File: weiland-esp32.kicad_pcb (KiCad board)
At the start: 2 copper layers, 20.2 x 58 mm, 22 parts, among them J1 S02B-PASK-2, J2 20021221-00006T4LF, J3 S02B-PASK-2, J4 S02B-PASK-2, J6 S02B-PASK-2, J7 S02B-PASK-2, U1 ESP32-WROOM-32E(8MB), U2 AMS1117-3.3_C347222, U3 GR6205-SOP-8, U4 MAX98357AEWL_T

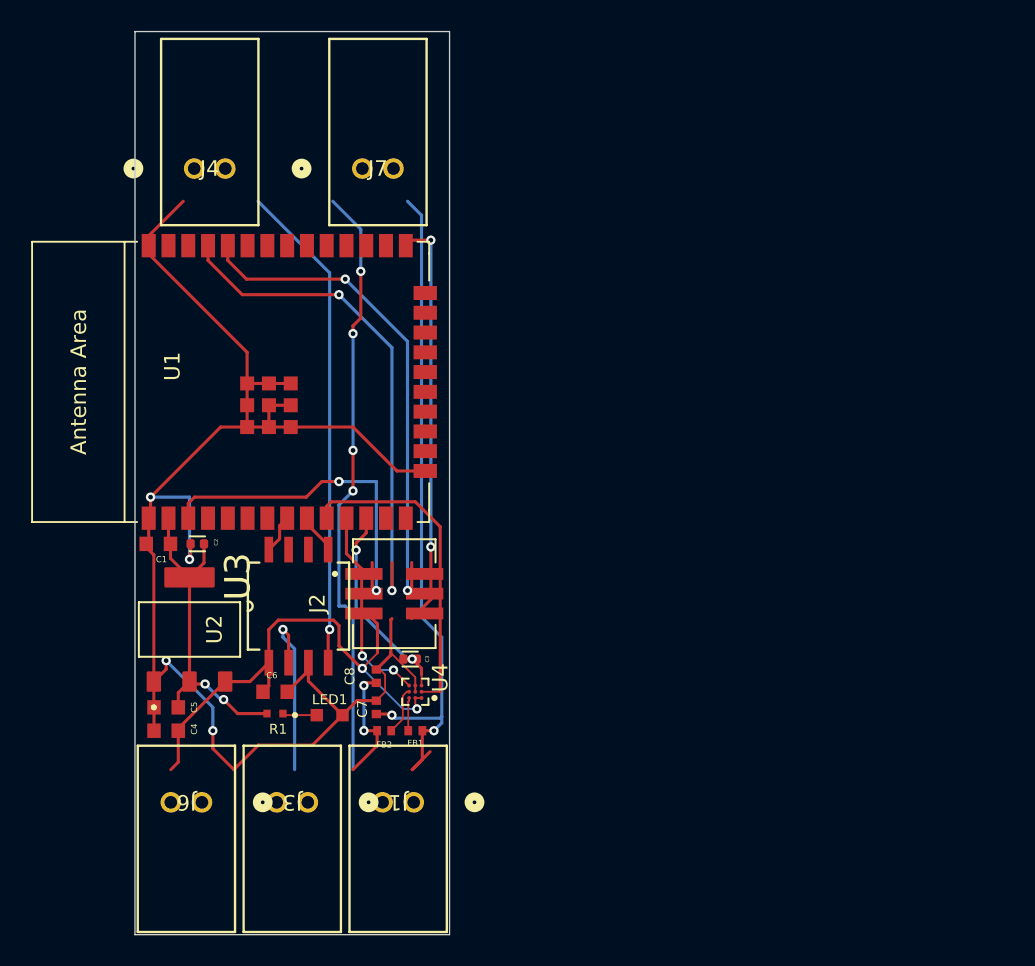
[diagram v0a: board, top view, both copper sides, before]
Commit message: good schematic before unshrouded header
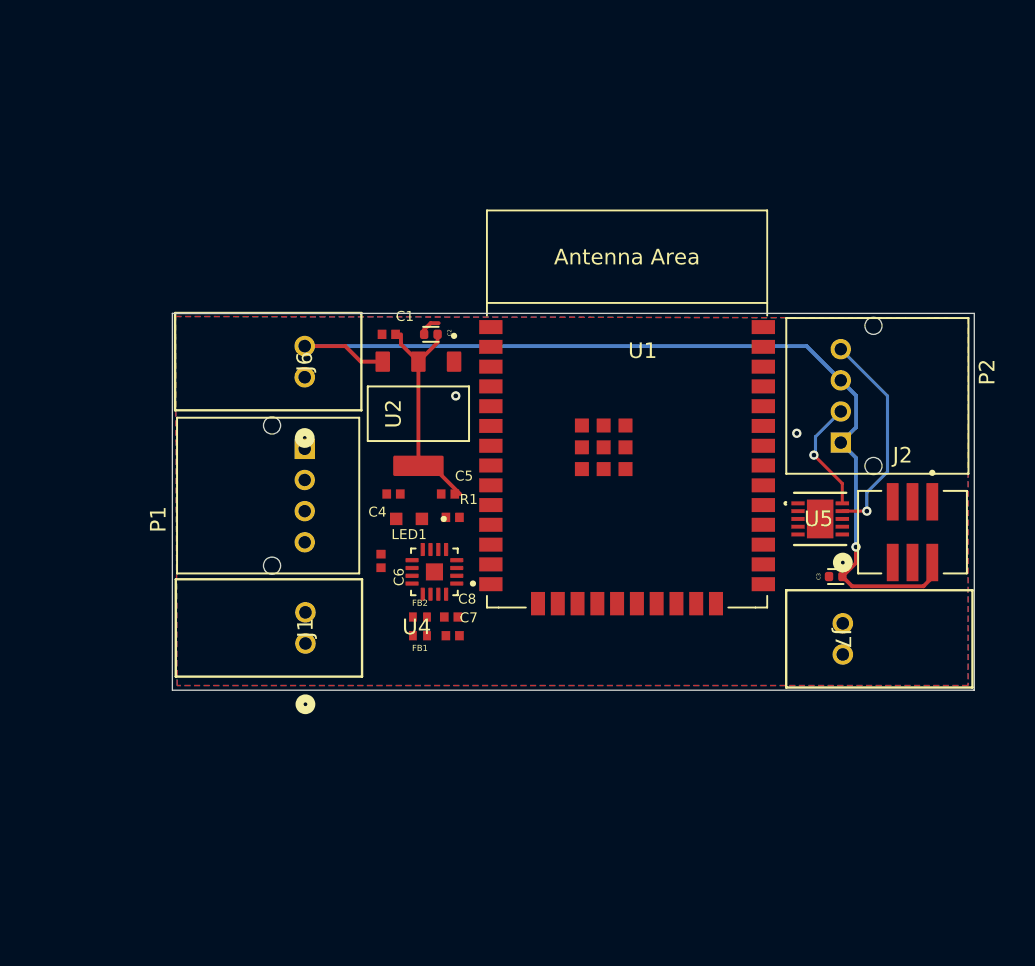
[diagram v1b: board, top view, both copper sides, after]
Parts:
- removed J3, J4: S02B-PASK-2, footprints:CONN2_S02B-PASK-2_JST
- removed U3: GR6205-SOP-8, motor_driver:SOP127P780X200-8N
- added P1: S04B-PASK-2_LF__SN_, S04B-PASK-2_LF__SN_:JST_S04B-PASK-2, F.Cu at (138.4, 99.9)
- added P2: S04B-PASK-2_LF__SN_, S04B-PASK-2_LF__SN_:JST_S04B-PASK-2, F.Cu at (172.8, 93.5)
- added U5: ULN2003F12FN-7, ULN2003:U-DFN3030-10_DIO, F.Cu at (171.5, 101.4)
- C1: footprint 22uF capacitor:CAPC1608X90N -> 100ohm-resistor:RESC1005X40N
- C4, C5: value 10uF -> 22uF; footprint 10 uF capacitor:CAPC1608X90N -> 100ohm-resistor:RESC1005X40N
- C6: footprint 10 uF capacitor:CAPC1608X90N -> 100ohm-resistor:RESC1005X40N
- C7, C8: footprint 220pF capacitor:CAPC1005X55N -> 100ohm-resistor:RESC1005X40N
- R1: value 5.1kΩ -> 100Ω; footprint 5-1-ohm-resistor:RES_ERJ2RKF5101X -> 100ohm-resistor:RESC1005X40N
- U4: footprint MAX98357AEWL_T:BGA9N40P3X3_134X143X69N -> MAX98357AETE_T:QFN50P300X300X80-17N
- moved J7 42.5 mm to (173.0, 108.1), turned to -90 degrees
- moved J2 33.5 mm to (177.4, 102.2), turned to 0 degrees
- moved J6 28.1 mm to (138.4, 92.3), turned to 90 degrees
- moved C3 27.8 mm to (172.5, 105.1), turned to 0 degrees
- moved U1 24.0 mm to (159.1, 96.1), turned to 0 degrees
- moved C5 22.7 mm to (147.6, 99.8)
- moved C4 21.1 mm to (144.1, 99.8), turned to 180 degrees
- moved U2 20.2 mm to (145.7, 94.6), turned to -90 degrees
- moved C2 20.2 mm to (146.5, 89.5)
- moved C1 20.0 mm to (143.8, 89.5)
- moved R1 17.0 mm to (147.9, 101.3), turned to 0 degrees
- moved LED1 13.6 mm to (145.1, 101.4), turned to 180 degrees
- moved J1 12.3 mm to (138.4, 109.4), turned to 90 degrees
- moved C6 10.8 mm to (143.3, 104.1), turned to -90 degrees
- moved U4 7.80 mm to (146.7, 104.8)
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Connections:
- U1 pad 10: /IO25 -> unconnected-(U1-IO25-Pad10)
- U1 pad 11: /IO26 -> unconnected-(U1-IO26-Pad11)
- U1 pad 12: /IO27 -> unconnected-(U1-IO27-Pad12)
- U1 pad 13: unconnected-(U1-IO14-Pad13) -> /IO14
- U1 pad 23: unconnected-(U1-IO15-Pad23) -> /IO15
- U1 pad 27: unconnected-(U1-IO16-Pad27) -> /IO16
- U1 pad 28: unconnected-(U1-IO17-Pad28) -> /IO17
- U1 pad 30: unconnected-(U1-IO18-Pad30) -> /IO18
- U1 pad 31: unconnected-(U1-IO19-Pad31) -> /IO19
- U1 pad 36: unconnected-(U1-IO22-Pad36) -> /IO22
- U1 pad 8: /IO32 -> unconnected-(U1-IO32-Pad8)
- U1 pad 9: /IO33 -> unconnected-(U1-IO33-Pad9)
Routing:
- net GND: track 104.8 -> 1.40 mm, vias 4 -> 2
- net /OUTN: track 46.2 -> 0.00 mm, vias 6 -> 0
- net /OUTP: track 44.6 -> 0.00 mm, vias 2 -> 0
- net /RXD0: track 32.6 -> 0.00 mm, vias 2 -> 0
- net /TXD0: track 32.5 -> 0.00 mm, vias 2 -> 0
- net +5V: track 32.4 -> 62.2 mm, vias 2 -> 1
- net /IO0: track 26.6 -> 0.00 mm, vias 2 -> 0
- net /OUTA: track 31.6 -> 7.37 mm
- net /EN: track 22.5 -> 0.00 mm, vias 2 -> 0
- net /IO25: track 20.6 -> 0.00 mm
- net /IO26: track 13.1 -> 0.00 mm, vias 2 -> 0
- net /IO27: track 13.0 -> 0.00 mm, vias 2 -> 0
- net +3V3: track 21.4 -> 13.7 mm, vias 2 -> 0
- net Net-(U4-OUTN): track 3.06 -> 0.00 mm
- net /IO33: track 2.58 -> 0.00 mm
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- added copper zone on B.Cu, net GND
- added copper zone on F.Cu, net GND
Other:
- board size 20.2 x 58 mm -> 51.5 x 24.2 mm
